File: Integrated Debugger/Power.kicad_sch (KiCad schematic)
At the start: 23 parts, among them J5 PWR, Q2 Generic N-MOSFET, SW3 Auxiliary Override, SW4 Target Override, U4 TPS7A2633DRVR, U5 TPS22914, U6 TPS22914

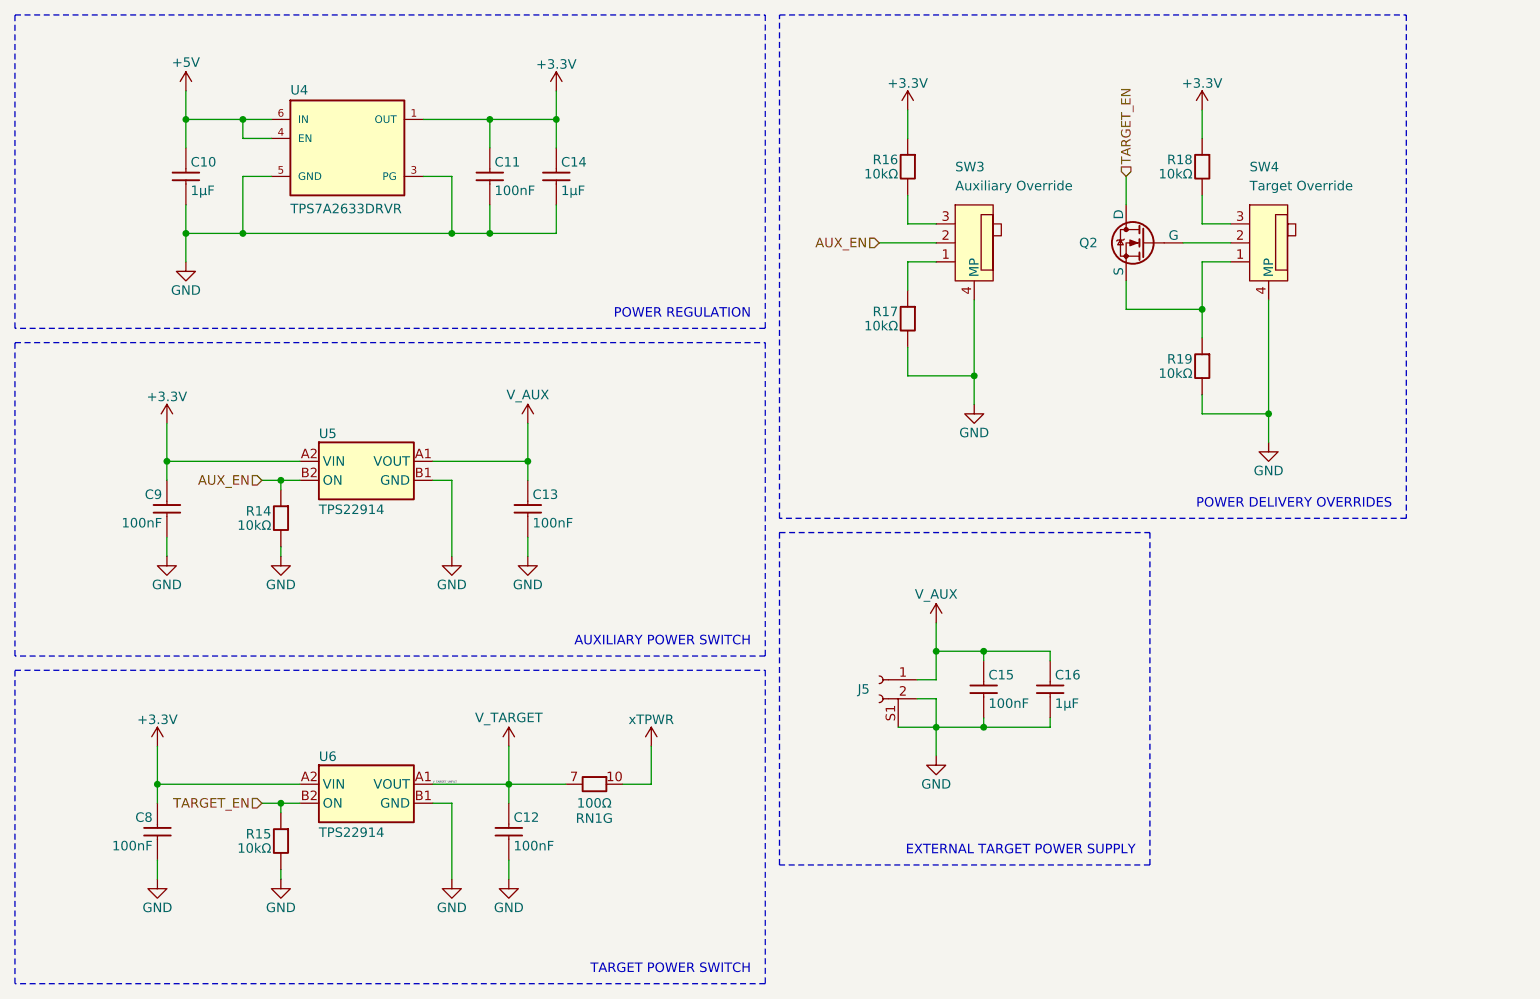
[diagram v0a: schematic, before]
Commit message: IDBG schematic
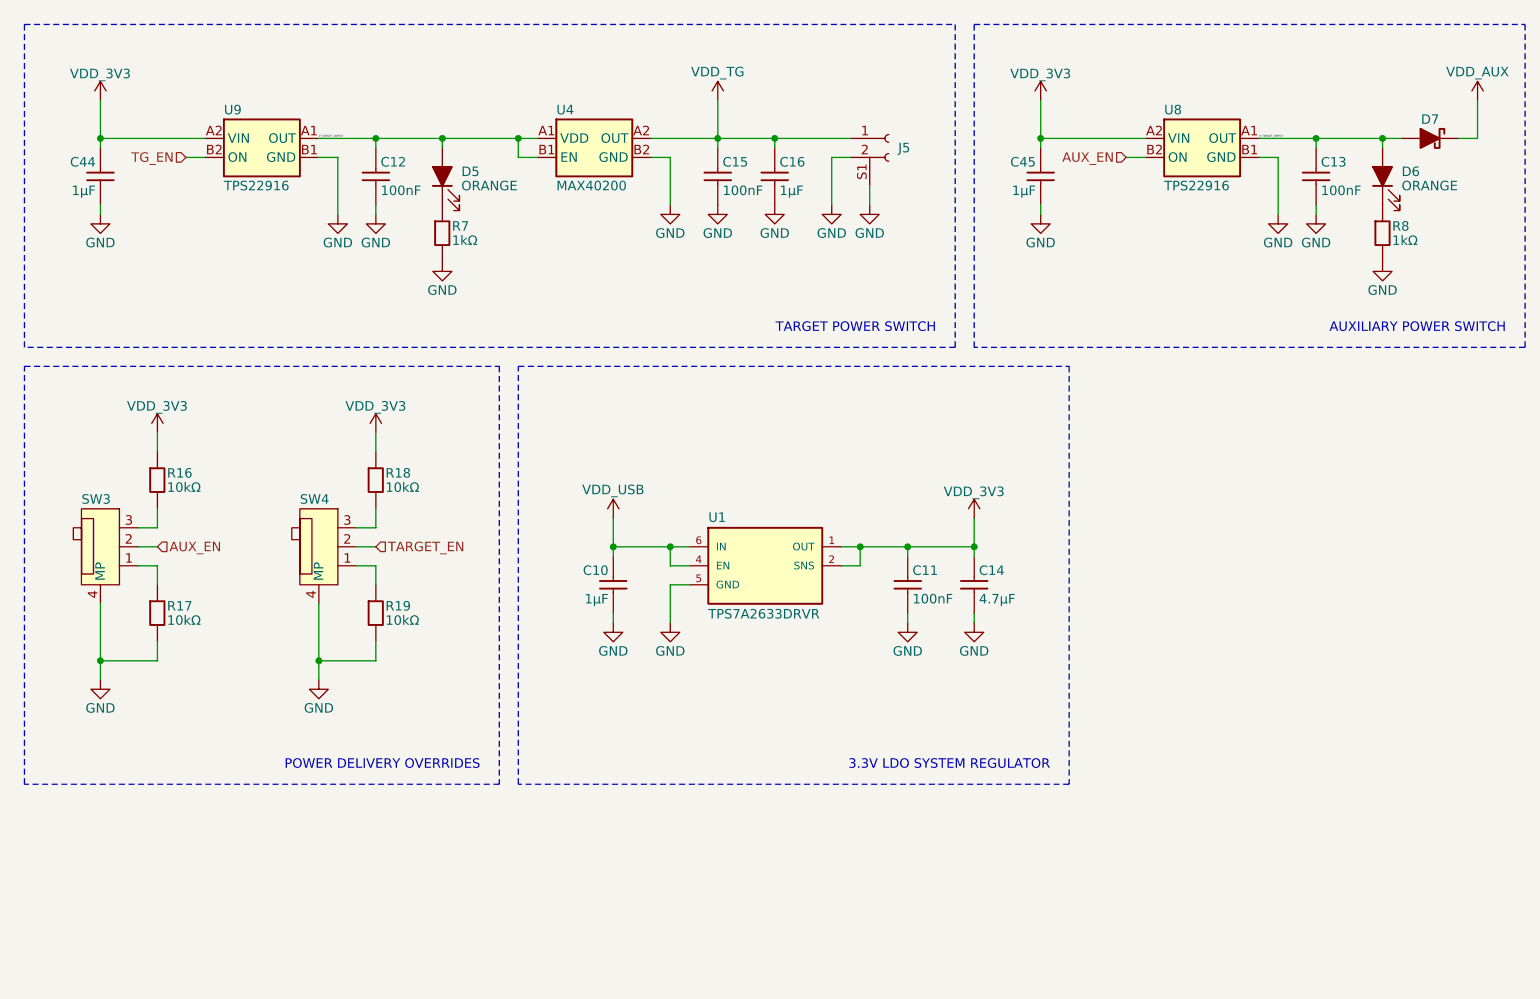
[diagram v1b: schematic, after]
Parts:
- removed C8, C9: 100nF, Picoballoon Passives:Capacitor 0201, symbol Picoballoon Passives:Capacitor
- removed Q2: Generic N-MOSFET, Picoballoon ICs:PICOSTAR-3_0.65, symbol Picoballoon ICs:Generic N-MOSFET
- removed R14, R15: 10kΩ, Picoballoon Passives:Resistor 0201, symbol Picoballoon Passives:Resistor
- removed RN1: 100Ω, Picoballoon Passives:Resistor 0402x8, symbol Picoballoon Passives:Resistor array 8
- removed U4: TPS7A2633DRVR, Picoballoon ICs:WSON-6 2x2mm, symbol Picoballoon ICs:LDO TPS7A26
- removed U5, U6: TPS22914, Picoballoon ICs:DSBGA-4, symbol Picoballoon ICs:TPS22914BYFPR
- added C44, C45: 1µF, Picoballoon Passives:Capacitor 0201, symbol Picoballoon Passives:Capacitor
- added D5, D6: ORANGE, Picoballoon Passives:LED 0201, symbol Picoballoon Passives:LED
- added D7: CFSH05-20L TR PBFREE, Picoballoon Passives:Diode SOD-882, symbol Picoballoon Passives:Schottky Diode
- added R7, R8: 1kΩ, Picoballoon Passives:Resistor 0201, symbol Picoballoon Passives:Resistor
- added U1: TPS7A2633DRVR, Picoballoon ICs:WSON-6 2x2mm, symbol Picoballoon ICs:LDO TLV767
- added U4: MAX40200, Picoballoon ICs:WLP-4, symbol Picoballoon ICs:MAX40200
- added U8, U9: TPS22916, Picoballoon ICs:DSBGA-4, symbol Picoballoon ICs:TPS22916CYFPR
- C10, C16: JLCPCB Part # C76930 -> (none)
- C11, C12, C13, C15: JLCPCB Part # C76934 -> (none)
- C14: value 1μF -> 4.7μF; JLCPCB Part # C76930 -> (none); LCSC Part # C335102 -> C335103; MPN GRM033R61C105ME15D -> GRM035R60J475ME15D
- J5: JLCPCB Part # C177225 -> (none); LCSC Part # C177225 -> C52995100; MPN 532610271 -> WAFA2-RDT1-2021-D
- R16, R17, R18, R19: JLCPCB Part # C717002 -> (none)
- SW3, SW4: JLCPCB Part # C2681570 -> (none)
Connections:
- net AUX_EN: now also U8.B2 (ON)
- net GND: now also C44.2, C45.2, R7.2, R8.2, U1.3 (GND), U1.5 (GND), U1.7 (EXP), U4.B2 (GND), U8.B1 (GND), U9.B1 (GND)
- net TARGET_EN: now also SW4.2
- net +3.3V renamed VDD_3V3
- net VDD_3V3: now also C44.1, C45.1, U1.1 (OUT), U1.2 (SNS), U8.A2 (VIN), U9.A2 (VIN)
- net +5V renamed VDD_USB
- net VDD_USB: now also U1.4 (EN), U1.6 (IN)
- net V_AUX renamed VDD_TG
- net VDD_TG: now also U4.A2 (OUT); no longer C13.1
- net V_TARGET renamed V_TARGET_UNFILT
- net V_TARGET_UNFILT: now also C13.1, D5.1 (K), D6.1 (K), D7.2 (A), U4.A1 (VDD), U4.B1 (EN), U8.A1 (OUT), U9.A1 (OUT)
- new net: D6.2 (A), R8.1
- new net: D5.2 (A), R7.1
- new net TG_EN: U9.B2 (ON)
- new net VDD_AUX: D7.1 (K)
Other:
- note added: "3.3V LDO SYSTEM REGULATOR"
- note removed: "EXTERNAL TARGET POWER SUPPLY"
- note removed: "POWER REGULATION"
- moved on the sheet: C10, C11, C12, C13, C14, C15, C16, J5, R16, R17, R18, R19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
